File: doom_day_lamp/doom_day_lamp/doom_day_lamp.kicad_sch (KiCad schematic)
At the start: 23 parts, among them J1 Conn_01x02_Female

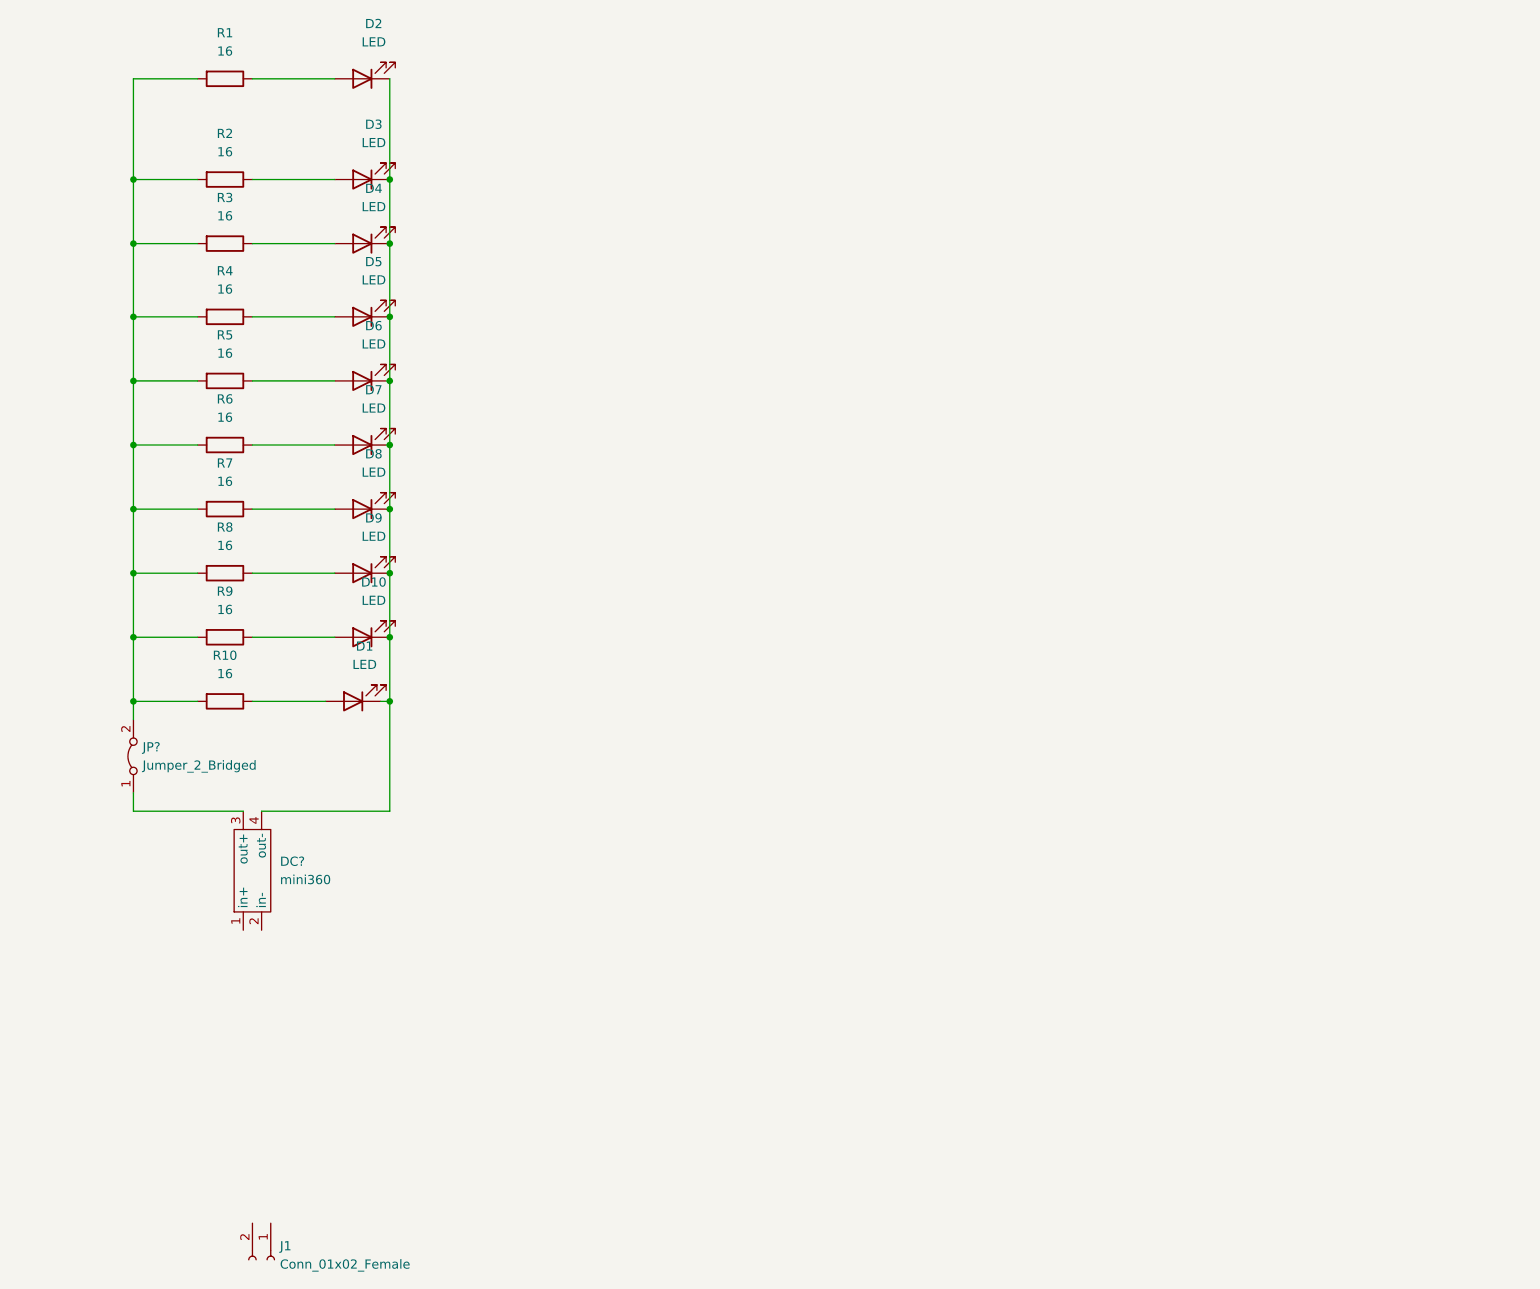
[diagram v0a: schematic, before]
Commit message: Add projects
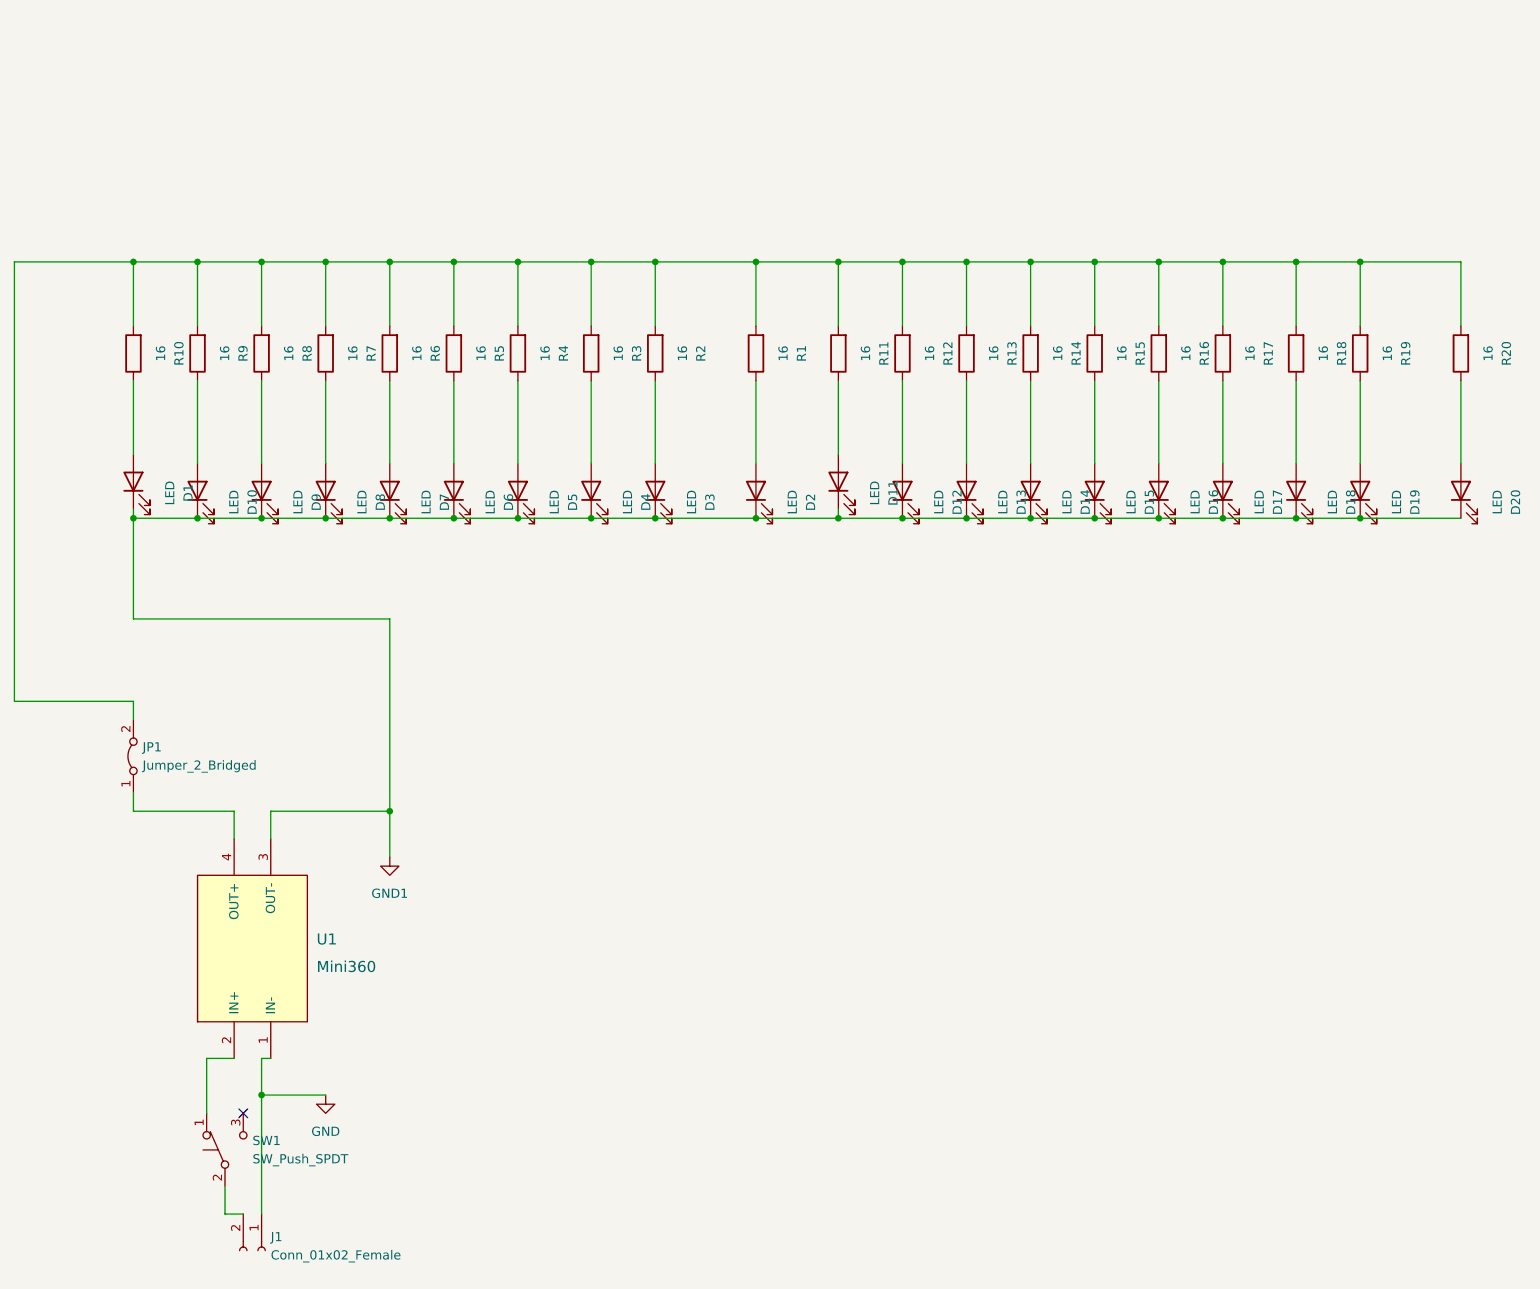
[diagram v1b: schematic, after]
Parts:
- removed DC?: mini360, symbol _dc_dc_converter:mini360
- added D11, D12, D13, D14, D15, D16, D17, D18, D19, D20: LED, LED_THT:LED_D3.0mm, symbol Device:LED
- added R11, R12, R13, R14, R15, R16, R17, R18, R19, R20: 16, Resistor_THT:R_Axial_DIN0207_L6.3mm_D2.5mm_P2.54mm_Vertical, symbol Device:R
- added SW1: SW_Push_SPDT, _switch:SW_CuK_OS102011MA1QN1_SPDT_Angled, symbol Switch:SW_Push_SPDT
- added U1: Mini360, _dc_dc_converters:Mini360_step-down, symbol _dc_dc_converter:Mini360
- J1: footprint Connector_AMASS:AMASS_XT30U-M_1x02_P5.0mm_Vertical -> Connector_PinHeader_2.00mm:PinHeader_1x02_P2.00mm_Vertical
- JP1: renamed from JP?; footprint (none) -> Connector_PinHeader_2.54mm:PinHeader_1x02_P2.54mm_Vertical
- R1, R10, R2, R3, R4, R5, R6, R7, R8, R9: footprint Resistor_THT:R_Axial_DIN0207_L6.3mm_D2.5mm_P7.62mm_Horizontal -> Resistor_THT:R_Axial_DIN0207_L6.3mm_D2.5mm_P2.54mm_Vertical
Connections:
- net GND1: now reaches D1.1 (K), D10.1 (K), D2.1 (K), D3.1 (K), D4.1 (K), D5.1 (K), D6.1 (K), D7.1 (K), D8.1 (K), D9.1 (K)
- net GND1: now also D11.1 (K), D12.1 (K), D13.1 (K), D14.1 (K), D15.1 (K), D16.1 (K), D17.1 (K), D18.1 (K), D19.1 (K), D20.1 (K), U1.3 (OUT-)
- net at JP1.2 (B), R1.2, R10.2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: now also R11.2, R12.2, R13.2, R14.2, R15.2, R16.2, R17.2, R18.2, R19.2, R20.2
- net GND: now reaches J1.1 (Pin_1)
- net GND: now also U1.1 (IN-)
- net at J1.2 (Pin_2): now also SW1.2 (B)
- net at JP1.1 (A): now also U1.4 (OUT+)
- new net: D15.2 (A), R15.1
- new net: D12.2 (A), R12.1
- new net: SW1.1 (A), U1.2 (IN+)
- new net: D20.2 (A), R20.1
- new net: D14.2 (A), R14.1
- new net: D19.2 (A), R19.1
- new net: D13.2 (A), R13.1
- new net: D16.2 (A), R16.1
- new net: D17.2 (A), R17.1
- new net: D11.2 (A), R11.1
- new net: D18.2 (A), R18.1
- no-connect marks 0 -> 1
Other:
- moved on the sheet: D1, D10, D2, D3, D4, D5, D6, D7, D8, D9, J1, R1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
